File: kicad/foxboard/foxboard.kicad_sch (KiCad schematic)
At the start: 183 parts, among them J2 USB_C_Receptacle_USB2.0, K1 KEYSW, K10 KEYSW, K11 KEYSW, K12 KEYSW, K13 KEYSW, K14 KEYSW, K15 KEYSW, K16 KEYSW, K17 KEYSW, K18 KEYSW, K19 KEYSW, K2 KEYSW, K20 KEYSW, K21 KEYSW, K22 KEYSW, K23 KEYSW, K24 KEYSW, K25 KEYSW, K26 KEYSW, K27 KEYSW, K28 KEYSW, K29 KEYSW, K3 KEYSW, K30 KEYSW, K31 KEYSW, K32 KEYSW, K33 KEYSW, K34 KEYSW, K35 KEYSW, K36 KEYSW, K37 KEYSW, K38 KEYSW, K39 KEYSW, K4 KEYSW, K40 KEYSW, K41 KEYSW, K42 KEYSW, K43 KEYSW, K44 KEYSW, K45 KEYSW, K46 KEYSW, K47 KEYSW, K48 KEYSW, K49 KEYSW, K5 KEYSW, K50 KEYSW, K51 KEYSW, K52 KEYSW, K53 KEYSW, K54 KEYSW, K55 KEYSW, K56 KEYSW, K57 KEYSW, K58 KEYSW, K59 KEYSW, K6 KEYSW, K60 KEYSW, K61 KEYSW, K62 KEYSW, K63 KEYSW, K64 KEYSW, K65 KEYSW, K66 KEYSW, K67 KEYSW, K68 KEYSW, K69 KEYSW, K7 KEYSW, K70 KEYSW, K71 KEYSW, K72 KEYSW, K73 KEYSW, K74 KEYSW, K75 KEYSW, K76 KEYSW, K77 KEYSW, K78 KEYSW, K79 KEYSW, K8 KEYSW, K80 KEYSW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

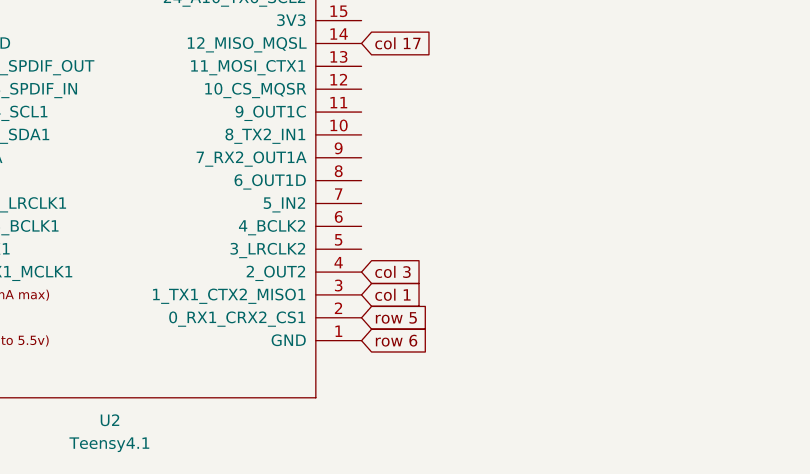
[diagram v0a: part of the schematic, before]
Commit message: fix
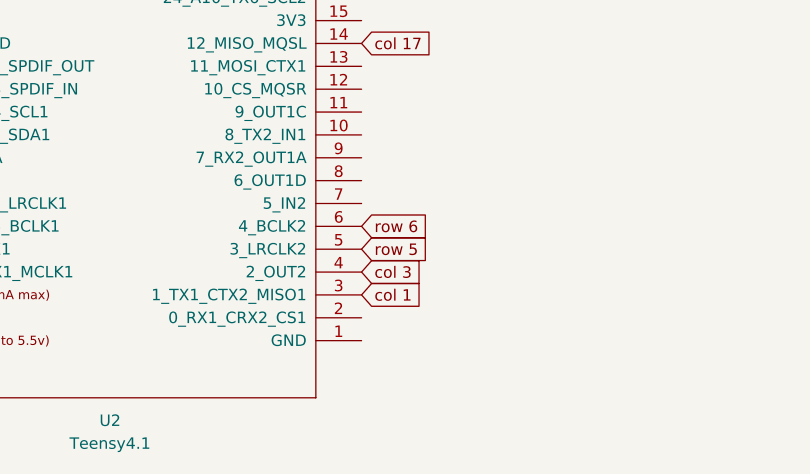
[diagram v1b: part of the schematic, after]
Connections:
- net row 5: now also U2.5 (3_LRCLK2); no longer U2.2 (0_RX1_CRX2_CS1)
- net row 6: now also U2.6 (4_BCLK2); no longer U2.1 (GND)

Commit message: wip v2
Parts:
- removed U2: Teensy4.1, teensy:Teensy41, symbol teensy:Teensy4.1
- added C1, C2: 10u, symbol Device:C
- added C10, C11, C12, C13, C5, C6, C7, C8, C9: 100n, symbol Device:C
- added C14, C3: 1u, symbol Device:C
- added C15, C4: C, symbol Device:C
- added C16, C17: 15p, symbol Device:C
- added J1: Conn_01x02, symbol Connector_Generic:Conn_01x02
- added R1, R2: 27.4, symbol Device:R
- added R3: 1k, symbol Device:R
- added R4: DNF, symbol Device:R
- added U1: RP2040, RP2040_minimal:RP2040-QFN-56, symbol MCU_RaspberryPi_RP2040:RP2040
- added U2: NCP1117-3.3_SOT223, Package_TO_SOT_SMD:SOT-223-3_TabPin2, symbol Regulator_Linear:NCP1117-3.3_SOT223
- added U3: W25Q128JVS, Package_SO:SOIC-8_5.3x5.3mm_P1.27mm, symbol Memory_Flash:W25Q128JVS
- added Y1: ABM8-272-T3, symbol Device:Crystal_GND24
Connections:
- net GND: now also C1.2, C10.2, C11.2, C12.2, C13.2, C14.2, C15.2, C16.1, C17.1, C2.1, C3.2, C4.2, C5.2, C6.2, C7.2, C8.2, C9.2, J1.1 (Pin_1), U2.1 (GND), U3.4 (GND), Y1.2 (G), Y1.4 (G)
- net VBUS: now also C1.1, U2.3 (VI)
- net col 1: now also U1.8 (GPIO6)
- net col 10: now also U1.18 (GPIO15)
- net col 11: now also U1.27 (GPIO16)
- net col 12: now also U1.28 (GPIO17)
- net col 13: now also U1.29 (GPIO18)
- net col 14: now also U1.30 (GPIO19)
- net col 15: now also U1.31 (GPIO20)
- net col 16: now also U1.32 (GPIO21)
- net col 17: now also U1.34 (GPIO22)
- net col 2: now also U1.9 (GPIO7)
- net col 3: now also U1.11 (GPIO8)
- net col 4: now also U1.12 (GPIO9)
- net col 5: now also U1.13 (GPIO10)
- net col 6: now also U1.14 (GPIO11)
- net col 7: now also U1.15 (GPIO12)
- net col 8: now also U1.16 (GPIO13)
- net col 9: now also U1.17 (GPIO14)
- net row 1: now also U1.2 (GPIO0)
- net row 2: now also U1.3 (GPIO1)
- net row 3: now also U1.4 (GPIO2)
- net row 4: now also U1.5 (GPIO3)
- net row 5: now also U1.6 (GPIO4)
- net row 6: now also U1.7 (GPIO5)
- net USB_D-: now reaches J2.A7 (D-), J2.B7 (D-)
- net USB_D-: now also R1.2
- net USB_D+: now reaches J2.A6 (D+), J2.B6 (D+)
- net USB_D+: now also R2.1
- new net: R3.1, R4.2, U3.1 (~{CS})
- new net: J1.2 (Pin_2), R3.2
- new net: R2.2, U1.46 (USB_DM)
- new net: R1.1, U1.47 (USB_DP)
- new net +1.1V: C3.1, C4.1, C5.1, U1.23 (DVDD), U1.45 (VREG_VOUT), U1.50 (DVDD)
- new net +3.3V: C10.1, C11.1, C12.1, C13.1, C14.1, C15.1, C2.2, C6.1, C7.1, C8.1, C9.1, R4.1, U1.1 (IOVDD), U1.10 (IOVDD), U1.22 (IOVDD), U1.33 (IOVDD), U1.42 (IOVDD), U1.43 (ADC_AVDD), U1.44 (VREG_IN), U1.48 (USB_VDD), U1.49 (IOVDD), U2.2 (VO), U3.8 (VCC)
- new net XIN: C17.2, U1.20 (XIN), Y1.1
- new net XOUT: C16.2, U1.21 (XOUT), Y1.3
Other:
- moved on the sheet: J2, R5, R6
